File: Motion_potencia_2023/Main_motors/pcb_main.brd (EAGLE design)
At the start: 200 x 180 mm, 22 parts, among them IC1 TEENSY_4.1, X5 5566-25569-2, X6 5566-25569-2, X7 5566-25569-2, X8 5566-25569-2

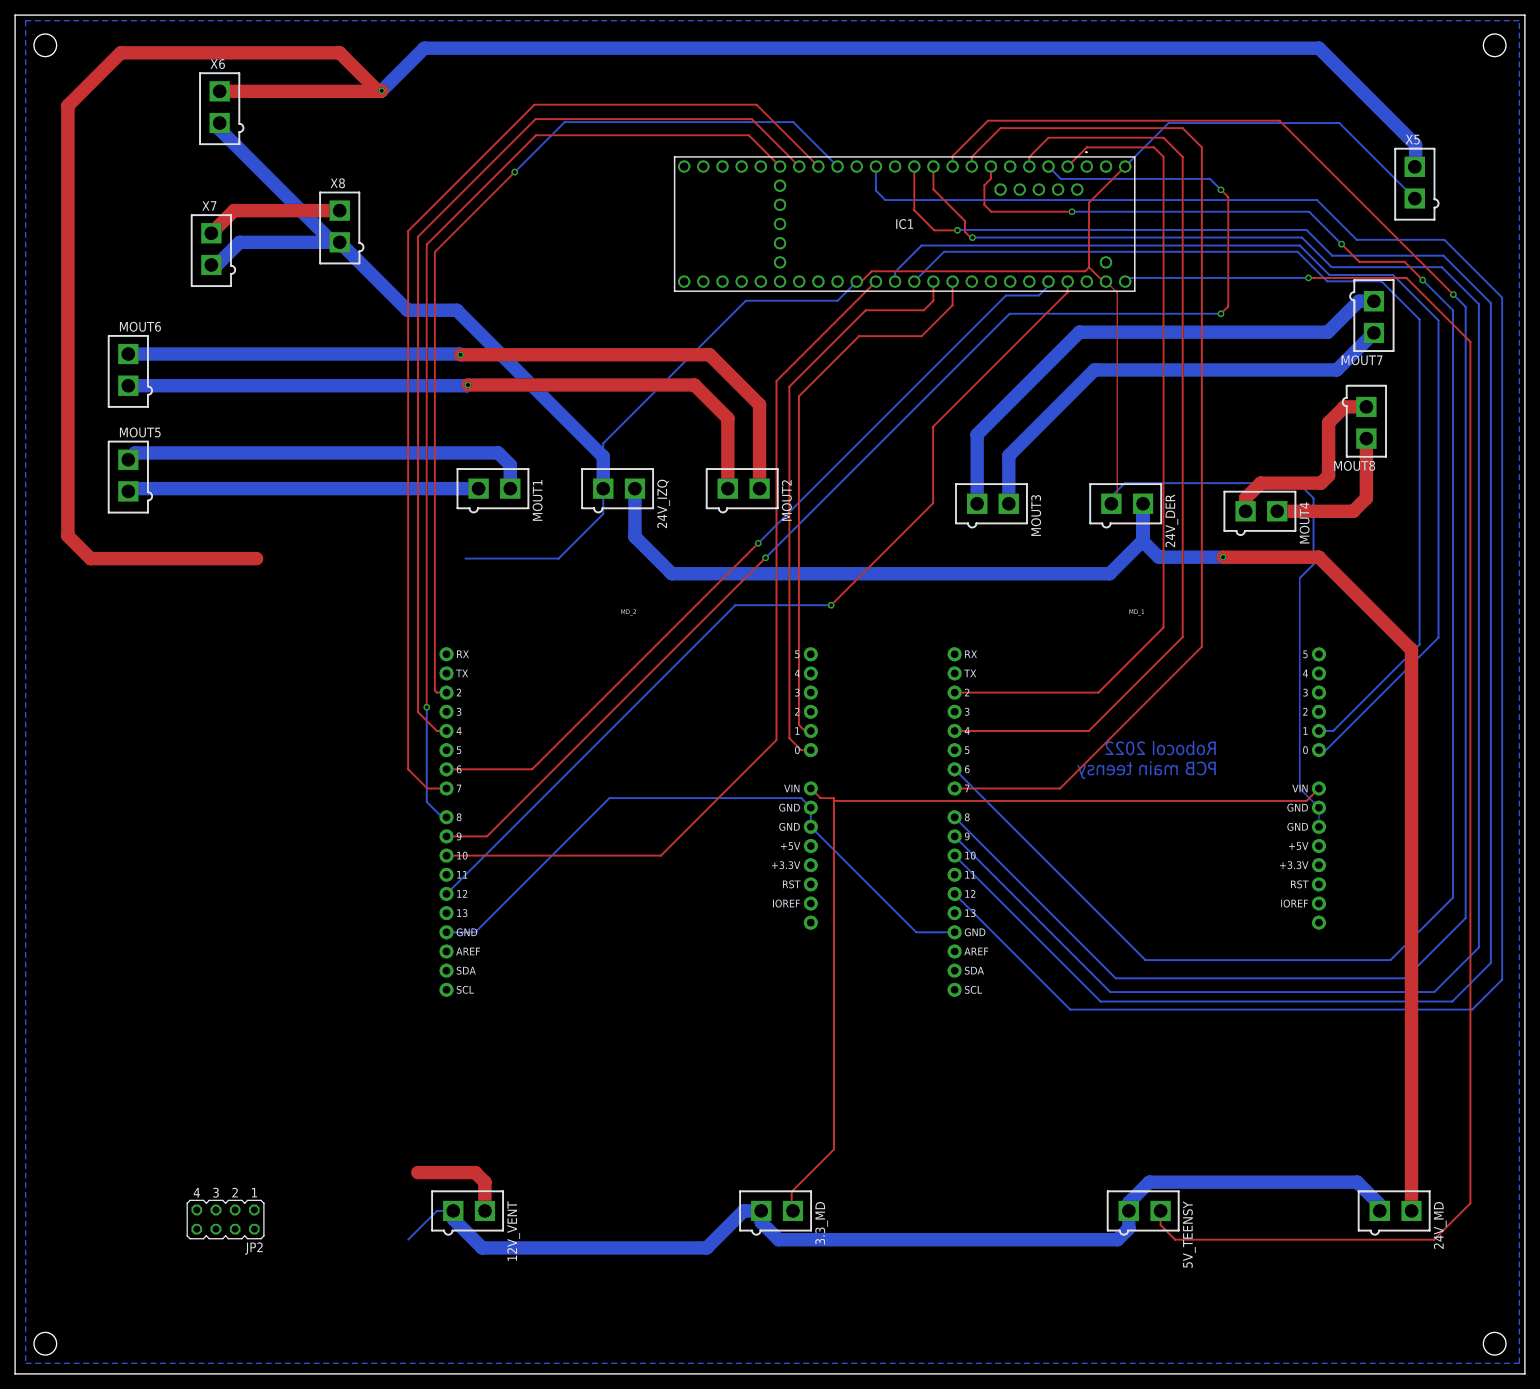
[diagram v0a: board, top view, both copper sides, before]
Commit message: main lista, sin revisión
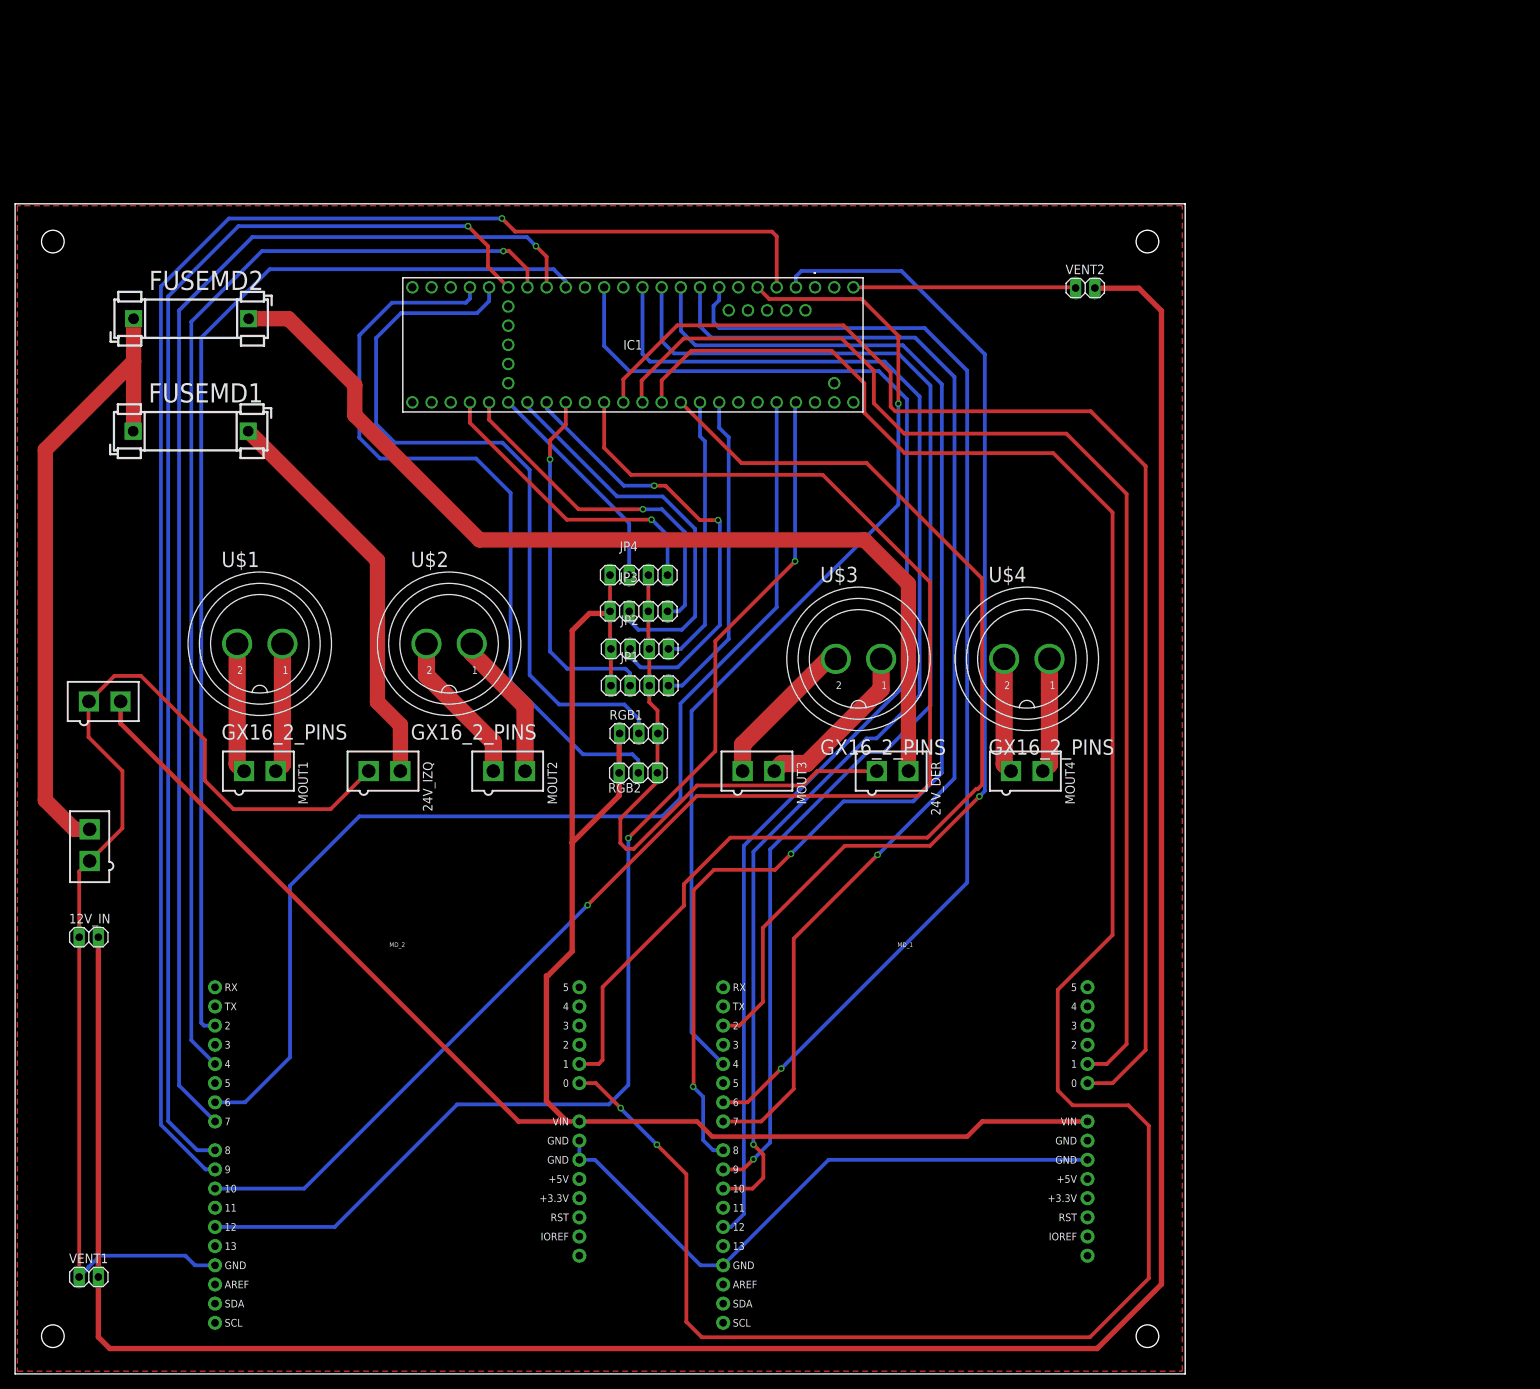
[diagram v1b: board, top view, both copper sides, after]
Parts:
- removed 12V_VENT, 3.3_MD, 5V_TEENSY, MOUT5, MOUT6, MOUT7, MOUT8, X5, X6, X7, X8: 5566-25569-2, molex_arreglado_2:5569-2
- added 12V_IN, VENT1, VENT2: (no value), pinhead:1X02
- added 5_MD: 5566-25569-2, molex_arreglado_2:5569-2
- added FUSEMD1, FUSEMD2: FUSEBLANK_5X20MM, fuse:FUSE_HOLDER_5X20MM
- added JP1, JP3, JP4: (no value), pinhead:1X04
- added RGB1, RGB2: (no value), pinhead:1X03
- added U$1, U$2, U$3, U$4: GX16_2_PINS, Robocol_Eagle_Libraries2:GX16_2_PINS_PADS
- JP2: device jumper:JP4Q -> pinhead:1X04
- moved 24V_MD 179.7 mm to (9.87, 70.0), turned to 0 degrees
- moved JP2 93.4 mm to (82.7, 96.0), turned to 0 degrees
- moved MD_1 53.7 mm to (117.9, 25.8)
- moved MD_2 53.7 mm to (50.6, 25.8)
- moved 24V_IZQ 48.6 mm to (48.9, 79.9)
- moved MOUT1 48.6 mm to (32.4, 79.9)
- moved MOUT2 48.6 mm to (65.4, 79.9)
- moved 24V_DER 47.1 mm to (116.2, 79.9)
- moved MOUT3 47.1 mm to (98.5, 79.9)
- moved MOUT4 46.4 mm to (134.0, 79.9)
- moved IC1 39.4 mm to (106.0, 143.9)
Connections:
- removed net 3.3V: JP2.7
- removed net 3.3V_MD: 3.3_MD.2, MD_1.VIN, MD_2.VIN
- removed net 5V_TEENSY: 5V_TEENSY.2, IC1.55
- removed net N$1: X7.2, X8.2
- removed net SCL_1: JP2.1
- removed net SCL_2: JP2.3
- removed net SDA_1: JP2.2
- removed net SDA_2: JP2.4
- new net 5V_MD: 5_MD.2, JP1.1, JP2.1, JP3.1, JP4.1, MD_1.VIN, MD_2.VIN, RGB1.1, RGB2.1
- new net A14: IC1.38, JP4.2
- new net A15: IC1.39, JP3.2
- new net A16: IC1.40, JP2.2
- new net A17: IC1.41, JP1.2
- new net D18: IC1.18, JP2.4
- new net D19: IC1.19, JP1.4
- new net D28: IC1.28, RGB1.2
- new net D29: IC1.29, RGB2.2
- new net D36: IC1.36, JP4.4
- new net D37: IC1.37, JP3.4
- new net FUSE20AMD1: 24V_IZQ.2, FUSEMD1.2
- new net FUSE20AMD2: 24V_DER.2, FUSEMD2.2
- net 12V_VENT: now also 12V_IN.2, VENT1.2, VENT2.2; no longer 12V_VENT.2, X5.2, X6.2
- net 24V_IN_MD: now also FUSEMD1.1, FUSEMD2.1; no longer 24V_DER.2, 24V_IZQ.2
- net GND: now also 12V_IN.1, 5_MD.1, JP1.3, JP2.3, JP3.3, JP4.3, RGB1.3, RGB2.3, VENT1.1, VENT2.1; no longer 12V_VENT.1, 3.3_MD.1, 5V_TEENSY.1, JP2.8, X5.1, X6.1, X7.1, X8.1
- net N$10: now also MOUT3.2, U$3.P$1; no longer MOUT4.2, MOUT8.2
- net N$3: now also U$1.P$2; no longer MOUT5.1
- net N$4: now also MOUT2.1, U$2.P$2; no longer MOUT1.2, MOUT5.2
- net N$5: now also MOUT2.2, U$2.P$1; no longer MOUT2.1, MOUT6.1
- net N$6: now also MOUT1.2, U$1.P$1; no longer MOUT2.2, MOUT6.2
- net N$7: now also MOUT4.1, U$4.P$2; no longer MOUT3.1, MOUT7.1
- net N$8: now also MOUT4.2, U$4.P$1; no longer MOUT3.2, MOUT7.2
- net N$9: now also MOUT3.1, U$3.P$2; no longer MOUT4.1, MOUT8.1
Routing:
- net 5V_MD: track 0.00 -> 260.3 mm
- net GND: track 592.6 -> 338.8 mm
- net CS_3: track 76.4 -> 293.3 mm, vias 0 -> 2
- net 5V_TEENSY: track 209.3 -> 0.00 mm, vias 1 -> 0
- net FUSE20AMD2: track 0.00 -> 129.1 mm
- net 3.3V_MD: track 125.6 -> 0.00 mm
- net 24V_IN_MD: track 203.2 -> 85.4 mm, vias 1 -> 0
- net D29: track 0.00 -> 102.7 mm
- net D28: track 0.00 -> 99.0 mm
- net M2_EN: track 262.9 -> 171.1 mm
- net PWM_2: track 255.9 -> 167.7 mm
- net PWM_1: track 248.1 -> 163.2 mm
- net PWM_4: track 116.2 -> 200.2 mm, vias 0 -> 1
- net N$6: track 97.5 -> 17.2 mm, vias 1 -> 0
- net CS_4: track 73.9 -> 152.9 mm
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- added copper zone on layer 1, net GND
- removed copper zone on layer 16, net GND
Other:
- board size 200 x 180 mm -> 155 x 155 mm
- board text removed: "Robocol 2022 PCB main teensy"
